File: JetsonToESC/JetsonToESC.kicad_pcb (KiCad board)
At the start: 2 copper layers, 42 x 47.2 mm, 35 parts, among them J1 Conn_01x12, J2 Conn_01x03, J3 Conn_01x02, U1 ESP32-C3_SUPERMINI_TH, U2 DS18B20, U3 LMR51420XDDCR, U4 MCP23018x-x-SS, U5 ACS759xCB-100B-PFF

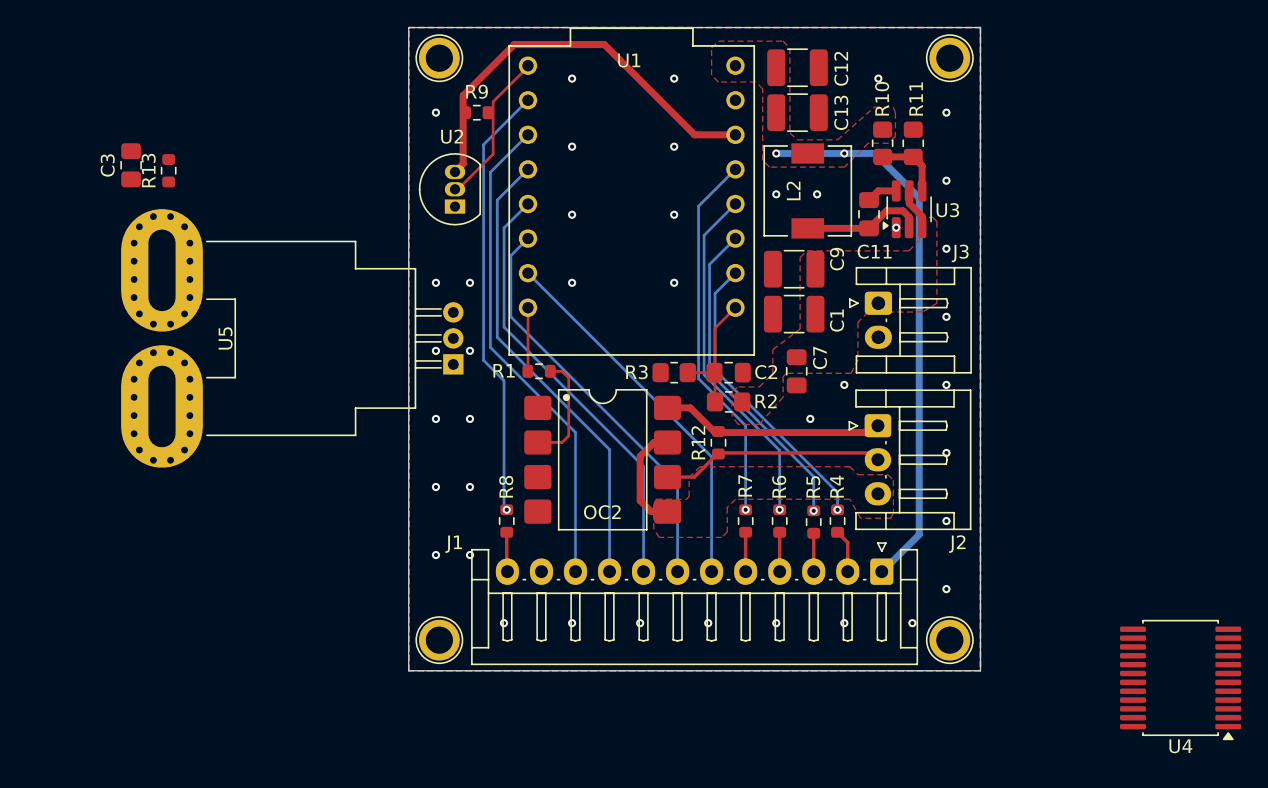
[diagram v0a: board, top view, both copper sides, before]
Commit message: Work on current sense and io expansion branch
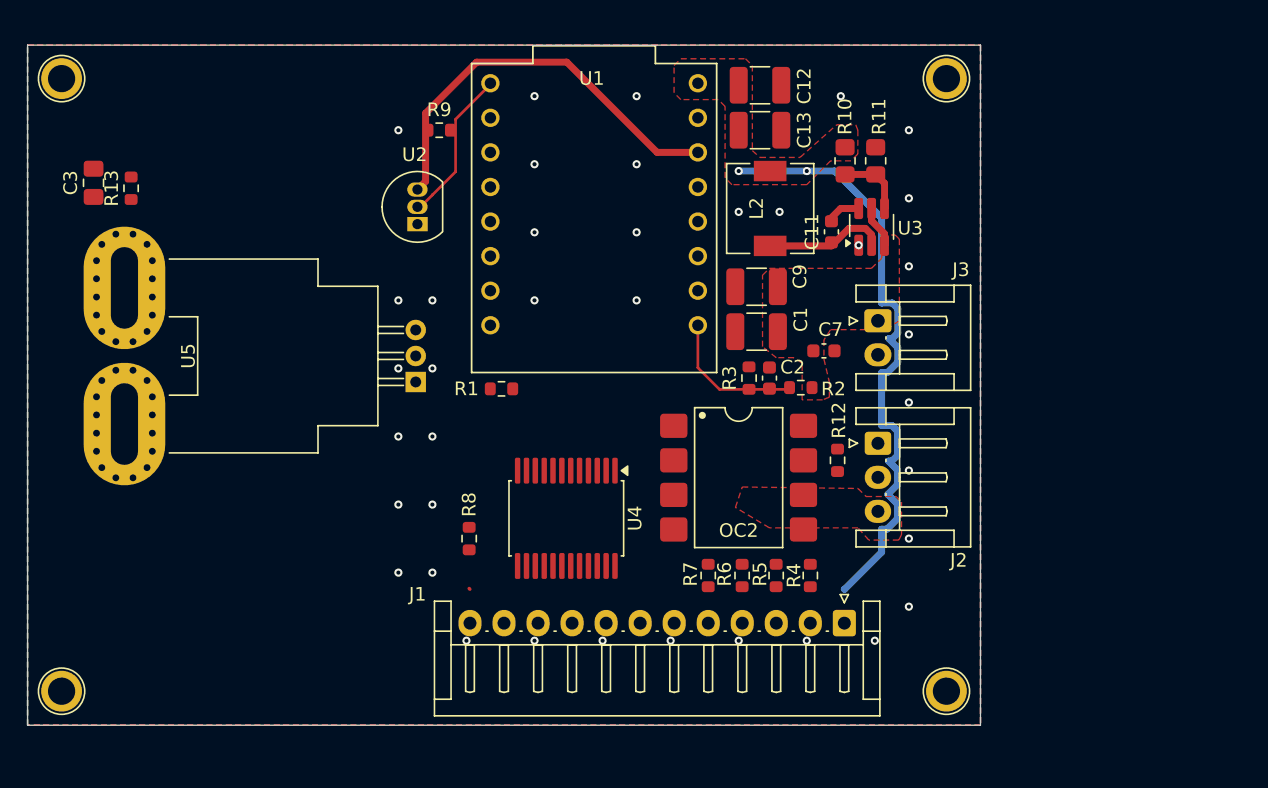
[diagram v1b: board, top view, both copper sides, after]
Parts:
- C11, C2, C7: footprint Capacitor_SMD:C_0805_2012Metric_Pad1.18x1.45mm_HandSolder -> Capacitor_SMD:C_0603_1608Metric
- R2, R3: footprint Resistor_SMD:R_0805_2012Metric_Pad1.20x1.40mm_HandSolder -> Resistor_SMD:R_0603_1608Metric
- moved U4 46.6 mm to (149.6, 114.8), turned to -90 degrees
- moved H3 28.0 mm to (112.5, 127.5)
- moved H1 27.8 mm to (112.5, 82.5)
- moved OC2 10.1 mm to (162.2, 111.8)
- moved R12 8.84 mm to (169.5, 110.5)
- moved R3 5.51 mm to (163.0, 104.5), turned to 90 degrees
- moved R2 5.40 mm to (166.8, 105.2)
- moved R6 4.86 mm to (162.5, 119.0)
- moved R7 4.85 mm to (160.0, 119.0)
- moved R5 4.80 mm to (165.0, 119.0)
- moved J1 4.68 mm to (170.0, 122.5)
- moved R4 4.47 mm to (167.5, 119.0)
- moved H4 3.76 mm to (177.5, 127.5)
- moved U2 3.05 mm to (138.6, 93.2)
- moved U5 3.05 mm to (138.5, 104.8)
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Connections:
- R4 pad 1: LED_BATT_LOW -> LED_OVERCURRENT
- R4 pad 2: Net-(U1-GPIO1) -> Net-(U4-GPB3)
- R5 pad 1: LED_BATT_MED -> LED_OVERCURRENT
- R5 pad 2: Net-(U1-GPIO2) -> Net-(U4-GPB4)
- R6 pad 2: Net-(U1-GPIO3) -> Net-(U4-GPB5)
- R7 pad 1: LED_OVERCURRENT -> LED_BATT_MED
- R7 pad 2: Net-(U1-GPIO4) -> Net-(U4-GPB6)
- R8 pad 1: LED_TEMP -> LED_BATT_LOW
- R8 pad 2: Net-(U1-GPIO6) -> Net-(U4-GPB7)
- U1 pad 1: Net-(U1-GPIO1) -> unconnected-(U1-GPIO1-Pad1)
- U1 pad 10: BUTTON_75% -> unconnected-(U1-GPIO10-Pad10)
- U1 pad 2: Net-(U1-GPIO2) -> unconnected-(U1-GPIO2-Pad2)
- U1 pad 20: BUTTON_100% -> unconnected-(U1-GPIO20-Pad20)
- U1 pad 3: Net-(U1-GPIO3) -> unconnected-(U1-GPIO3-Pad3)
- U1 pad 4: Net-(U1-GPIO4) -> unconnected-(U1-GPIO4-Pad4)
- U1 pad 6: Net-(U1-GPIO6) -> unconnected-(U1-GPIO6-Pad6)
- U1 pad 7: BUTTON_STOP -> unconnected-(U1-GPIO7-Pad7)
- U1 pad 8: BUTTON_25% -> I2C_SDA
- U1 pad 9: BUTTON_50% -> I2C_SCL
- U4 pad 5: LED_OVERCURRENT -> Net-(U4-GPB3)
- U4 pad 6: LED_OVERCURRENT -> Net-(U4-GPB4)
- U4 pad 7: LED_BATT_HI -> Net-(U4-GPB5)
- U4 pad 8: LED_BATT_MED -> Net-(U4-GPB6)
- U4 pad 9: LED_BATT_LOW -> Net-(U4-GPB7)
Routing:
- net BUTTON_STOP: track 36.8 -> 0.00 mm
- net BUTTON_25%: track 34.4 -> 0.00 mm
- net BUTTON_50%: track 33.0 -> 0.00 mm
- net Net-(U1-GPIO6): track 32.2 -> 0.00 mm, vias 1 -> 0
- net BUTTON_75%: track 30.3 -> 0.00 mm
- net BUTTON_100%: track 28.6 -> 0.00 mm
- net Net-(U1-GPIO4): track 27.6 -> 0.00 mm, vias 1 -> 0
- net Net-(U1-GPIO3): track 25.7 -> 0.00 mm, vias 1 -> 0
- net Net-(U1-GPIO2): track 24.0 -> 0.00 mm, vias 1 -> 0
- net Net-(U1-GPIO1): track 21.9 -> 0.00 mm, vias 1 -> 0
- net VBEC: track 16.4 -> 0.00 mm
- net ESC_PWM: track 16.4 -> 0.00 mm
- net Net-(OC2-Pad2): track 8.27 -> 0.00 mm
- net GNDB: track 8.25 -> 0.00 mm
- net 5V: track 40.5 -> 45.6 mm
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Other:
- board size 42 x 47.2 mm -> 70 x 50 mm
